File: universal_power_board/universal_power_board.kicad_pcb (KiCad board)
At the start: 2 copper layers, 77 x 75 mm, 100 parts, among them J1 Pixhawk Power, J10 5V OUTPUT, J11 BATT OUTPUT, J12 BATT OUTPUT, J2 BATT INPUT, J3 BATT OUTPUT, J4 5V OUTPUT, J5 5V OUTPUT, J6 BATT OUTPUT, J7 5V OUTPUT, J8 5V OUTPUT, J9 5V OUTPUT, U1 OKL-T_6-W12N-C

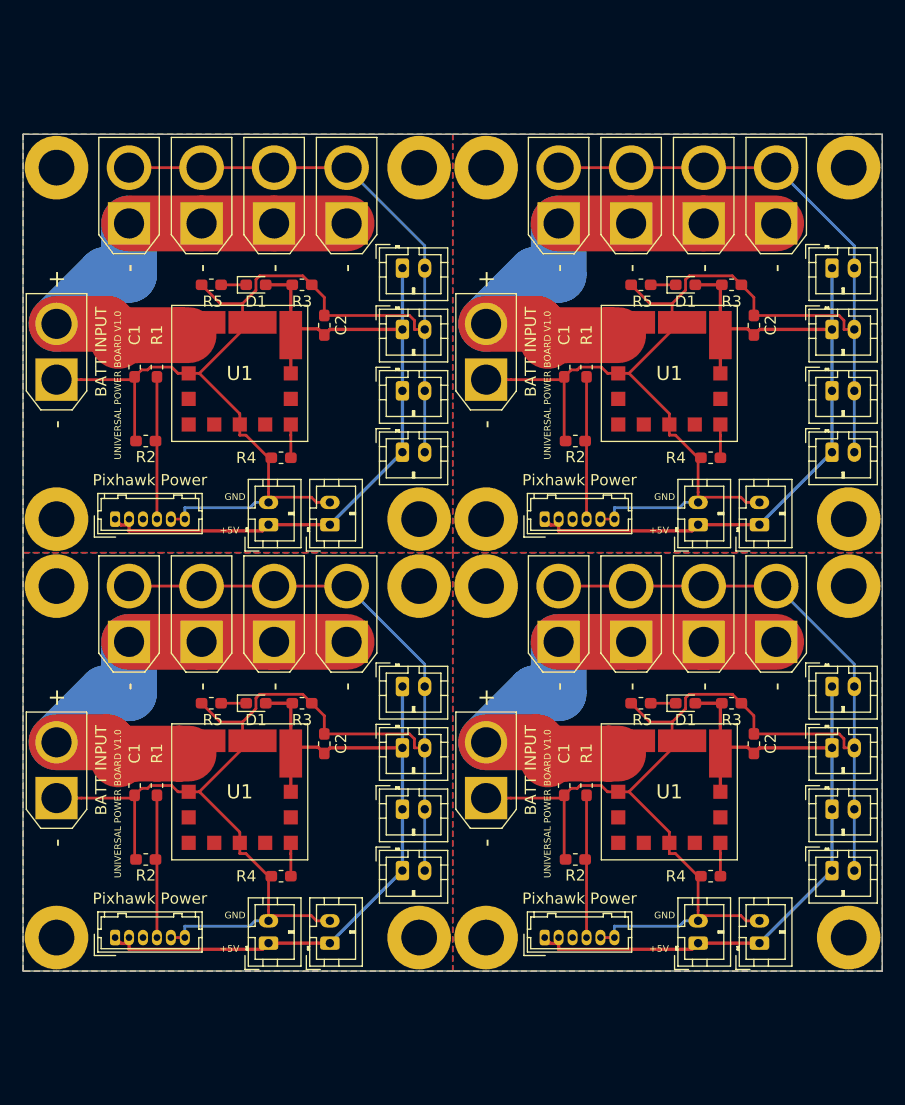
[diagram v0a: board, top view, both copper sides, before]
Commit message: update v1.1
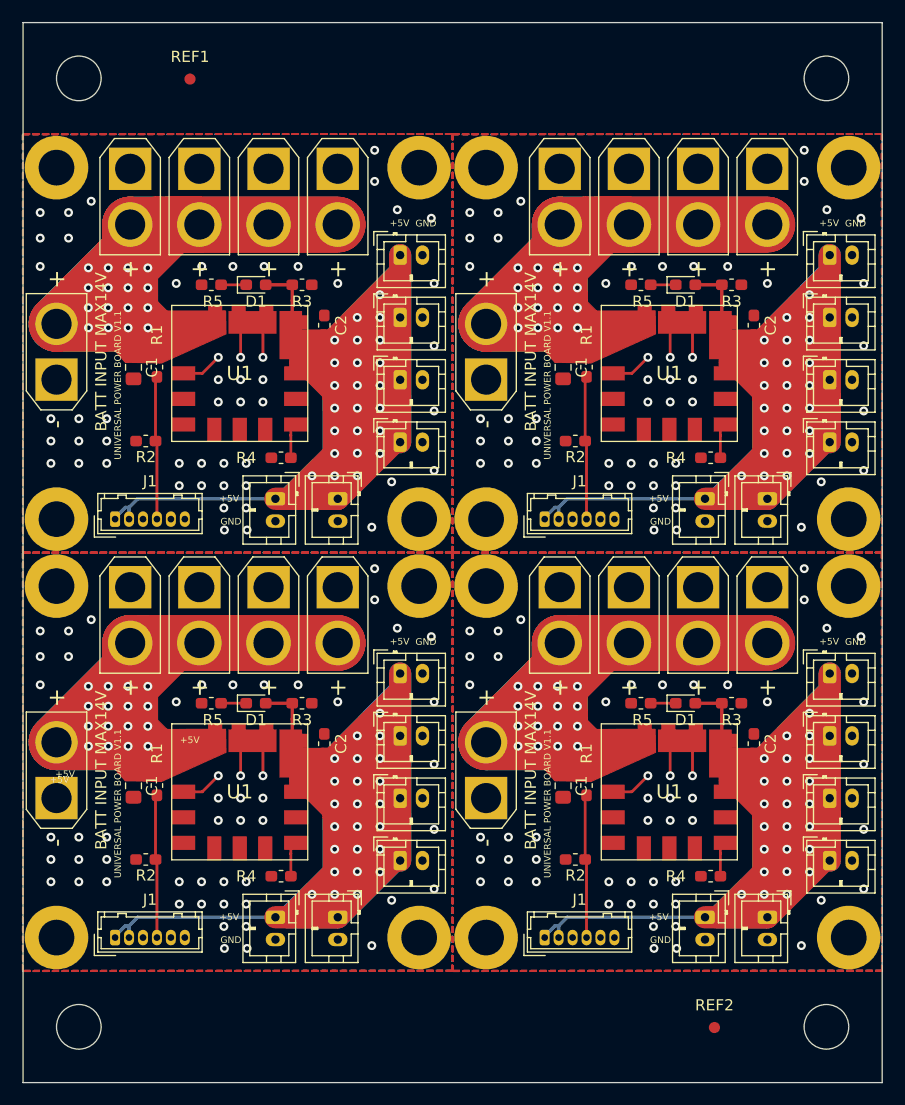
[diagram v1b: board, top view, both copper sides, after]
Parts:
- removed the C1 at (160.5, 132.4)
- removed the C1 at (122.0, 132.4)
- removed the C1 at (160.5, 94.9)
- removed the C1 at (122.0, 94.9)
- removed the J10 at (184.5, 140.0)
- removed the J10 at (146.0, 140.0)
- removed the J10 at (184.5, 102.5)
- removed the J10 at (146.0, 102.5)
- removed the J11 at (173.0, 119.5)
- removed the J11 at (134.5, 119.5)
- removed the J11 at (173.0, 82.0)
- removed the J12 at (179.5, 119.5)
- removed the J12 at (141.0, 119.5)
- removed the J12 at (179.5, 82.0)
- removed the J3 at (166.5, 119.5)
- removed the J3 at (128.0, 119.5)
- removed the J3 at (166.5, 82.0)
- removed the J4 at (184.5, 129.0)
- removed the J4 at (146.0, 129.0)
- removed the J4 at (184.5, 91.5)
- removed the J4 at (146.0, 91.5)
- removed the J5 at (184.5, 134.5)
- removed the J5 at (146.0, 134.5)
- removed the J5 at (184.5, 97.0)
- removed the J5 at (146.0, 97.0)
- removed the J6 at (160.0, 119.5)
- removed the J6 at (121.5, 119.5)
- removed the J6 at (160.0, 82.0)
- removed the J7 at (172.5, 146.5)
- removed the J7 at (134.0, 146.5)
- removed the J7 at (172.5, 109.0)
- removed the J7 at (134.0, 109.0)
- removed the J8 at (178.0, 146.5)
- removed the J8 at (139.5, 146.5)
- removed the J8 at (178.0, 109.0)
- removed the J8 at (139.5, 109.0)
- removed the J9 at (184.5, 123.5)
- removed the J9 at (146.0, 123.5)
- removed the J9 at (184.5, 86.0)
- removed the J9 at (146.0, 86.0)
- added C1: 22uF 25V, Inductor_SMD:L_0805_2012Metric_Pad1.15x1.40mm_HandSolder, F.Cu at (160.4, 132.4)
- added C1: 22uF 25V, Inductor_SMD:L_0805_2012Metric_Pad1.15x1.40mm_HandSolder, F.Cu at (121.9, 132.4)
- added C1: 22uF 25V, Inductor_SMD:L_0805_2012Metric_Pad1.15x1.40mm_HandSolder, F.Cu at (160.4, 94.9)
- added C1: 22uF 25V, Inductor_SMD:L_0805_2012Metric_Pad1.15x1.40mm_HandSolder, F.Cu at (121.9, 94.9)
- added J10: 5V OUTPUT, Connector_JST:JST_PH_B2B-PH-K_1x02_P2.00mm_Vertical, F.Cu at (178.7, 144.2)
- added J10: 5V OUTPUT, Connector_JST:JST_PH_B2B-PH-K_1x02_P2.00mm_Vertical, F.Cu at (140.2, 144.2)
- added J10: 5V OUTPUT, Connector_JST:JST_PH_B2B-PH-K_1x02_P2.00mm_Vertical, F.Cu at (178.7, 106.7)
- added J10: 5V OUTPUT, Connector_JST:JST_PH_B2B-PH-K_1x02_P2.00mm_Vertical, F.Cu at (140.2, 106.7)
- added J11: BATT OUTPUT, Connector_AMASS:AMASS_XT30U-F_1x02_P5.0mm_Vertical, F.Cu at (172.5, 114.6)
- added J11: BATT OUTPUT, Connector_AMASS:AMASS_XT30U-F_1x02_P5.0mm_Vertical, F.Cu at (134.0, 114.6)
- added J11: BATT OUTPUT, Connector_AMASS:AMASS_XT30U-F_1x02_P5.0mm_Vertical, F.Cu at (172.5, 77.1)
- added J12: BATT OUTPUT, Connector_AMASS:AMASS_XT30U-F_1x02_P5.0mm_Vertical, F.Cu at (178.7, 114.6)
- added J12: BATT OUTPUT, Connector_AMASS:AMASS_XT30U-F_1x02_P5.0mm_Vertical, F.Cu at (140.2, 114.6)
- added J12: BATT OUTPUT, Connector_AMASS:AMASS_XT30U-F_1x02_P5.0mm_Vertical, F.Cu at (178.7, 77.1)
- added J3: BATT OUTPUT, Connector_AMASS:AMASS_XT30U-F_1x02_P5.0mm_Vertical, F.Cu at (166.3, 114.6)
- added J3: BATT OUTPUT, Connector_AMASS:AMASS_XT30U-F_1x02_P5.0mm_Vertical, F.Cu at (127.8, 114.6)
- added J3: BATT OUTPUT, Connector_AMASS:AMASS_XT30U-F_1x02_P5.0mm_Vertical, F.Cu at (166.3, 77.1)
- added J4: 5V OUTPUT, Connector_JST:JST_PH_B2B-PH-K_1x02_P2.00mm_Vertical, F.Cu at (184.3, 122.3)
- added J4: 5V OUTPUT, Connector_JST:JST_PH_B2B-PH-K_1x02_P2.00mm_Vertical, F.Cu at (145.8, 122.3)
- added J4: 5V OUTPUT, Connector_JST:JST_PH_B2B-PH-K_1x02_P2.00mm_Vertical, F.Cu at (184.3, 84.8)
- added J4: 5V OUTPUT, Connector_JST:JST_PH_B2B-PH-K_1x02_P2.00mm_Vertical, F.Cu at (145.8, 84.8)
- added J5: 5V OUTPUT, Connector_JST:JST_PH_B2B-PH-K_1x02_P2.00mm_Vertical, F.Cu at (184.3, 127.9)
- added J5: 5V OUTPUT, Connector_JST:JST_PH_B2B-PH-K_1x02_P2.00mm_Vertical, F.Cu at (145.8, 127.9)
- added J5: 5V OUTPUT, Connector_JST:JST_PH_B2B-PH-K_1x02_P2.00mm_Vertical, F.Cu at (184.3, 90.4)
- added J5: 5V OUTPUT, Connector_JST:JST_PH_B2B-PH-K_1x02_P2.00mm_Vertical, F.Cu at (145.8, 90.4)
- added J6: BATT OUTPUT, Connector_AMASS:AMASS_XT30U-F_1x02_P5.0mm_Vertical, F.Cu at (160.1, 114.6)
- added J6: BATT OUTPUT, Connector_AMASS:AMASS_XT30U-F_1x02_P5.0mm_Vertical, F.Cu at (121.6, 114.6)
- added J6: BATT OUTPUT, Connector_AMASS:AMASS_XT30U-F_1x02_P5.0mm_Vertical, F.Cu at (160.1, 77.1)
- added J7: 5V OUTPUT, Connector_JST:JST_PH_B2B-PH-K_1x02_P2.00mm_Vertical, F.Cu at (184.3, 133.5)
- added J7: 5V OUTPUT, Connector_JST:JST_PH_B2B-PH-K_1x02_P2.00mm_Vertical, F.Cu at (145.8, 133.5)
- added J7: 5V OUTPUT, Connector_JST:JST_PH_B2B-PH-K_1x02_P2.00mm_Vertical, F.Cu at (184.3, 96.0)
- added J7: 5V OUTPUT, Connector_JST:JST_PH_B2B-PH-K_1x02_P2.00mm_Vertical, F.Cu at (145.8, 96.0)
- added J8: 5V OUTPUT, Connector_JST:JST_PH_B2B-PH-K_1x02_P2.00mm_Vertical, F.Cu at (184.3, 139.1)
- added J8: 5V OUTPUT, Connector_JST:JST_PH_B2B-PH-K_1x02_P2.00mm_Vertical, F.Cu at (145.8, 139.1)
- added J8: 5V OUTPUT, Connector_JST:JST_PH_B2B-PH-K_1x02_P2.00mm_Vertical, F.Cu at (184.3, 101.6)
- added J8: 5V OUTPUT, Connector_JST:JST_PH_B2B-PH-K_1x02_P2.00mm_Vertical, F.Cu at (145.8, 101.6)
- added J9: 5V OUTPUT, Connector_JST:JST_PH_B2B-PH-K_1x02_P2.00mm_Vertical, F.Cu at (173.1, 144.2)
- added J9: 5V OUTPUT, Connector_JST:JST_PH_B2B-PH-K_1x02_P2.00mm_Vertical, F.Cu at (134.6, 144.2)
- added J9: 5V OUTPUT, Connector_JST:JST_PH_B2B-PH-K_1x02_P2.00mm_Vertical, F.Cu at (173.1, 106.7)
- added J9: 5V OUTPUT, Connector_JST:JST_PH_B2B-PH-K_1x02_P2.00mm_Vertical, F.Cu at (134.6, 106.7)
- added REF1: Fiducial_1mm_Mask2mm, Fiducial:Fiducial_1mm_Mask2mm, F.Cu at (127.0, 69.1)
- added REF2: Fiducial_1mm_Mask2mm, Fiducial:Fiducial_1mm_Mask2mm, F.Cu at (174.0, 154.1)
- J2 (x4): value BATT INPUT -> BATT INPUT MAX14V
- moved J12 4.96 mm to (140.2, 77.1), turned to 270 degrees
- moved J11 4.93 mm to (134.0, 77.1), turned to 270 degrees
- moved J3 4.90 mm to (127.8, 77.1), turned to 270 degrees
- moved J6 4.90 mm to (121.6, 77.1), turned to 270 degrees
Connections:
- J11 pad 1: +BATT -> GND
- J11 pad 2: GND -> +BATT
- J12 pad 1: +BATT -> GND
- J12 pad 2: GND -> +BATT
- J3 pad 1: +BATT -> GND
- J3 pad 2: GND -> +BATT
- J6 pad 1: +BATT -> GND
- J6 pad 2: GND -> +BATT
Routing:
- net +5V: track 268.8 -> 813.1 mm, vias 0 -> 100
- net GND: track 527.2 -> 43.9 mm, vias 0 -> 208
- net +BATT: track 206.8 -> 639.8 mm, vias 0 -> 64
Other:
- board size 77 x 75 mm -> 77 x 95 mm
- board text added: "UNIVERSAL POWER BOARD V1.1"
- board text removed: "UNIVERSAL POWER BOARD V1.0"
